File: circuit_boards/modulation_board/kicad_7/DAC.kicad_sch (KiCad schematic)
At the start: 4 parts

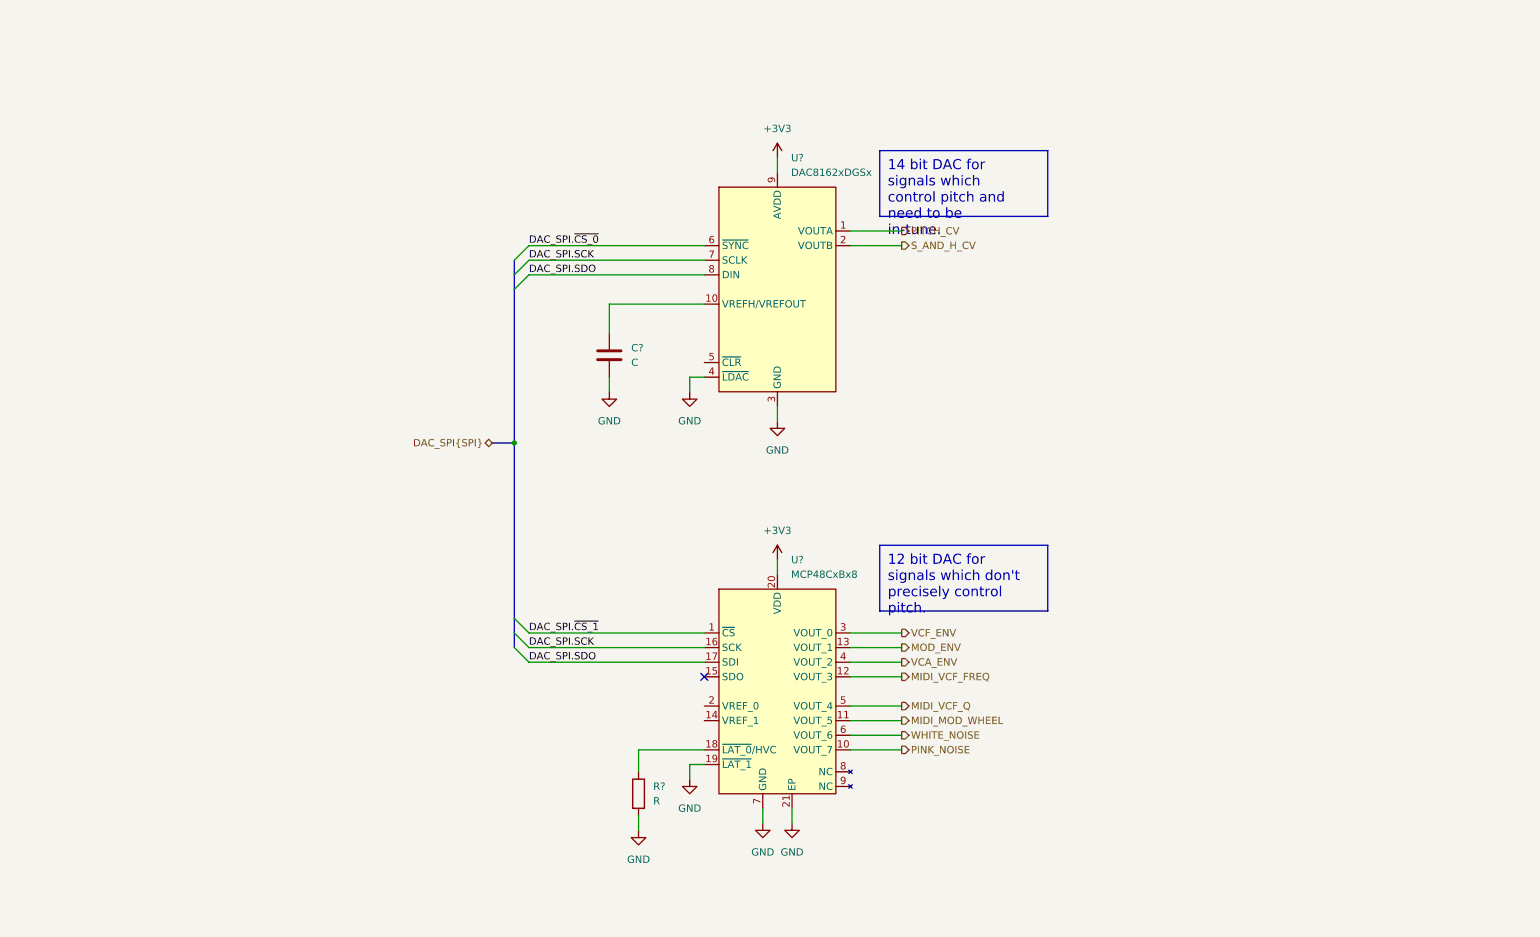
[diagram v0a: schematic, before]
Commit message: Progress on circuit boards
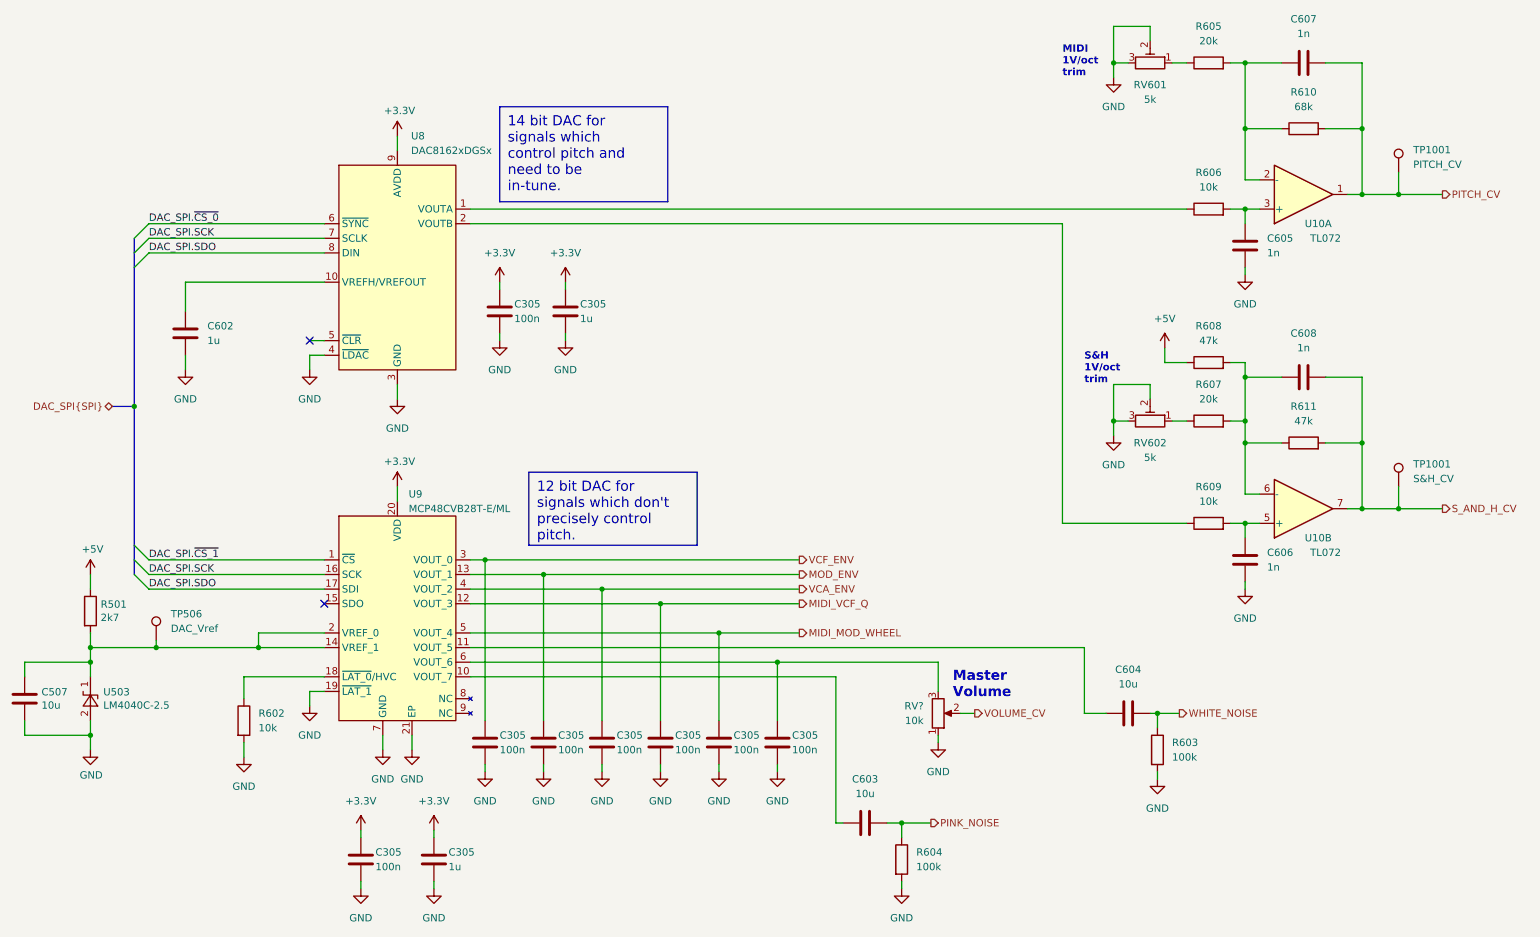
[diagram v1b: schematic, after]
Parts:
- added C305 (x2): 1u, Capacitor_SMD:C_0805_2012Metric, symbol Device:C
- added C305 (x8): 100n, Capacitor_SMD:C_0603_1608Metric, symbol Device:C
- added C507, C603, C604: 10u, Capacitor_SMD:C_0805_2012Metric, symbol Device:C
- added C605, C606, C607, C608: 1n, Capacitor_SMD:C_0603_1608Metric, symbol Device:C
- added R501: 2k7, Resistor_SMD:R_0603_1608Metric, symbol Device:R
- added R603, R604: 100k, Resistor_SMD:R_0603_1608Metric, symbol Device:R
- added R605, R607: 20k, Resistor_SMD:R_0603_1608Metric, symbol Device:R
- added R606, R609: 10k, Resistor_SMD:R_0603_1608Metric, symbol Device:R
- added R608, R611: 47k, Resistor_SMD:R_0603_1608Metric, symbol Device:R
- added R610: 68k, Resistor_SMD:R_0603_1608Metric, symbol Device:R
- added RV601, RV602: 5k, Potentiometer_THT:Potentiometer_Bourns_3296W_Vertical, symbol Device:R_Potentiometer_Trim
- added RV?: 10k, Potentiometer_THT:Potentiometer_Alpha_RD901F-40-00D_Single_Vertical, symbol Device:R_Potentiometer
- added TP1001: S&H_CV, TestPoint:TestPoint_Keystone_5000-5004_Miniature, symbol Connector:TestPoint
- added TP1001: PITCH_CV, TestPoint:TestPoint_Keystone_5000-5004_Miniature, symbol Connector:TestPoint
- added TP506: DAC_Vref, TestPoint:TestPoint_Keystone_5000-5004_Miniature, symbol Connector:TestPoint
- added U10: TL072, Package_SO:SOIC-8_3.9x4.9mm_P1.27mm, symbol Amplifier_Operational:TL072
- added U503: LM4040C-2.5, Package_TO_SOT_SMD:SOT-23, symbol Reference_Voltage:LM4040DBZ-2.5
- C602: renamed from C?; value C -> 1u; footprint (none) -> Capacitor_SMD:C_0805_2012Metric
- R602: renamed from R?; value R -> 10k; footprint (none) -> Resistor_SMD:R_0603_1608Metric
- U9: renamed from U?; value MCP48CxBx8 -> MCP48CVB28T-E/ML; footprint Package_DFN_QFN:QFN-20-1EP_4x4mm_P0.5mm_EP2.7x2.7mm_ThermalVias -> Package_DFN_QFN:QFN-20-1EP_4x4mm_P0.5mm_EP2.7x2.7mm
- gave numbers to parts that had none: 1
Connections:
- net MIDI_VCF_FREQ is gone; now on net MIDI_VCF_Q: U9.12 (VOUT_3)
- net GND: now also C305.2, C305.2, C305.2, C305.2, C305.2, C305.2, C305.2, C305.2, C305.2, C305.2, C507.2, C605.1, C606.1, R603.2, R604.2, RV601.2, RV601.3, RV602.2, RV602.3, RV?.1, U503.2 (A)
- net MIDI_MOD_WHEEL: now also U9.5 (VOUT_4), C305.1; no longer U9.11 (VOUT_5)
- net MIDI_VCF_Q: now also C305.1; no longer U9.5 (VOUT_4)
- net MOD_ENV: now also C305.1
- net PINK_NOISE: now also C603.2, R604.1; no longer U9.10 (VOUT_7)
- net PITCH_CV: now also C607.2, R610.2, TP1001.1, U10.1; no longer U8.1 (VOUTA)
- net S_AND_H_CV: now also C608.2, R611.2, TP1001.1, U10.7; no longer U8.2 (VOUTB)
- net VCA_ENV: now also C305.1
- net VCF_ENV: now also C305.1
- net WHITE_NOISE: now also C604.2, R603.1; no longer U9.6 (VOUT_6)
- net at U9.14 (VREF_1): now also U9.2 (VREF_0), C507.1, R501.2, TP506.1, U503.1 (K)
- net +3V3 renamed +3.3V
- net +3.3V: now also C305.1, C305.1, C305.1, C305.1
- new net: C603.1, U9.10 (VOUT_7)
- new net: C604.1, U9.11 (VOUT_5)
- new net: C305.1, RV?.3, U9.6 (VOUT_6)
- new net: C606.2, R609.2, U10.5 (+)
- new net: R607.1, RV602.1
- new net: C608.1, R607.2, R608.2, R611.1, U10.6 (-)
- new net: C607.1, R605.2, R610.1, U10.2 (-)
- new net: C605.2, R606.2, U10.3 (+)
- new net: R606.1, U8.1 (VOUTA)
- new net: R605.1, RV601.1
- new net: R609.1, U8.2 (VOUTB)
- new net +5V: R501.1, R608.1
- new net VOLUME_CV: RV?.2
- no-connect marks 1 -> 2
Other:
- note added: "MIDI 1V/oct trim"
- note added: "Master Volume"
- note added: "S&H 1V/oct trim"
- moved on the sheet: C602, R602, U8, U9
